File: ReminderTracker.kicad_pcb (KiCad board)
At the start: 2 copper layers, 92 x 150 mm, 23 parts, among them J1 External RTC, SW1 SW_Push, SW2 SW_Push, SW3 SW_Push, SW4 SW_Push, SW5 SW_Push, SW6 SW_Push, U1 XIAO-ESP32-C3-DIP

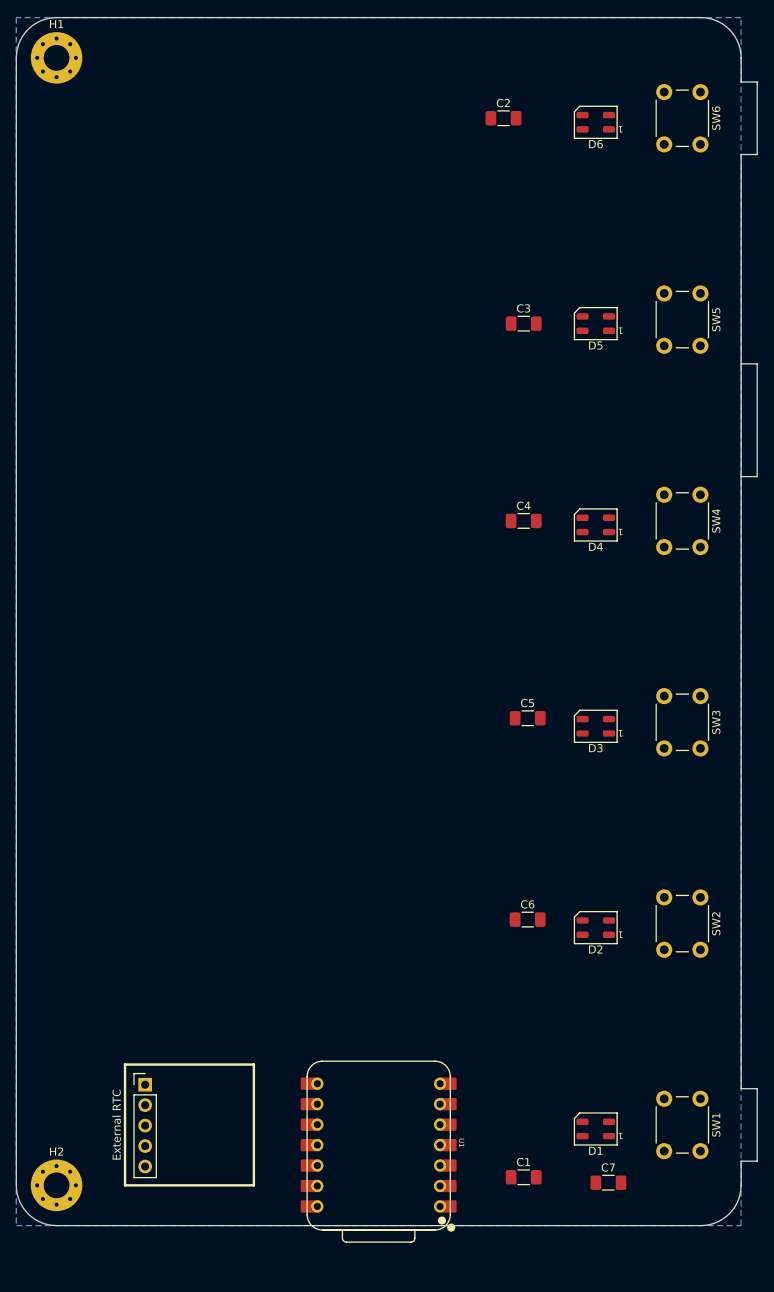
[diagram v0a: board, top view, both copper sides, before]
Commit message: R1
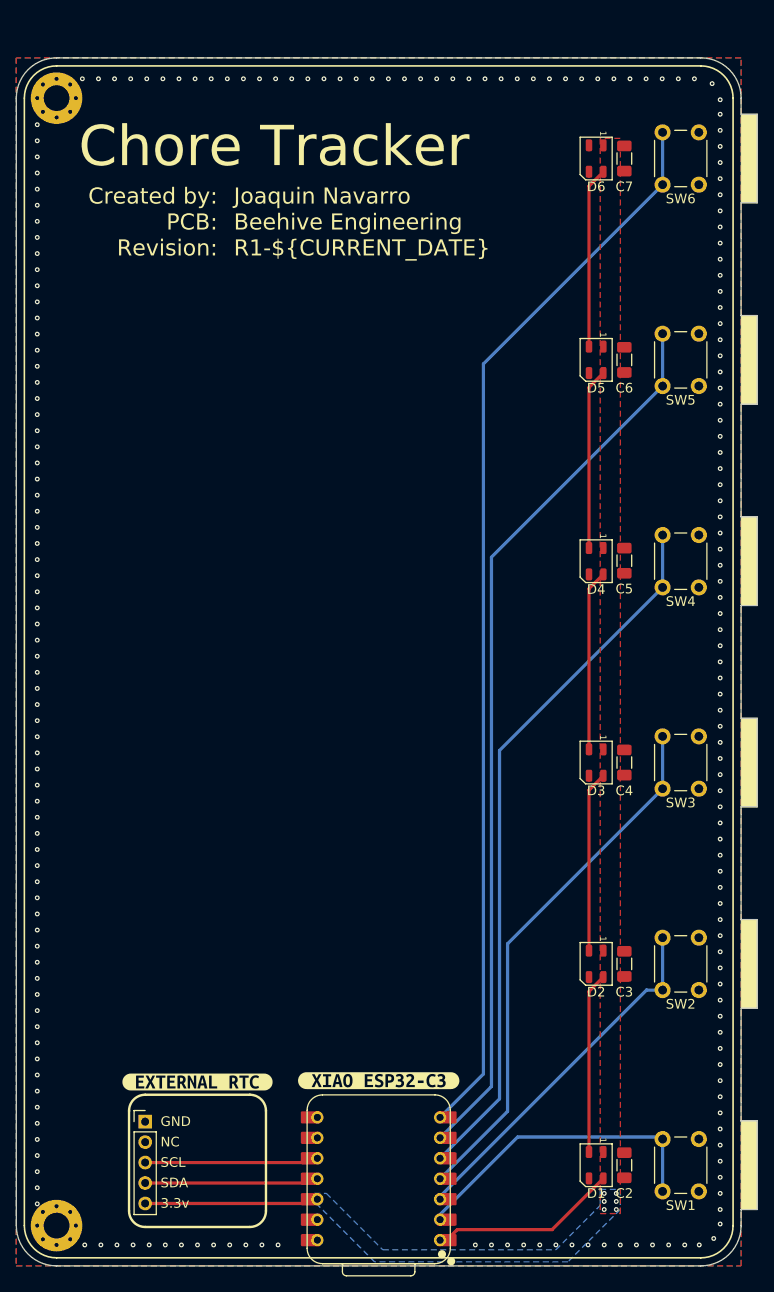
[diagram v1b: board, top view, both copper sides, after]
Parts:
- removed C1: 100pF, Capacitor_SMD:C_1206_3216Metric_Pad1.33x1.80mm_HandSolder
- added kibuzzard-69BB9782: G***, kibuzzard-69BB9782, F.Cu at (77.5, 157.2)
- added kibuzzard-69BB979E: G***, kibuzzard-69BB979E, F.Cu at (100.0, 157.0)
- moved C2 130.9 mm to (130.5, 167.5), turned to -90 degrees
- moved C7 127.2 mm to (130.5, 42.5), turned to -90 degrees
- moved C3 80.5 mm to (130.5, 142.5), turned to -90 degrees
- moved C6 70.5 mm to (130.5, 67.5), turned to -90 degrees
- moved C4 32.5 mm to (130.5, 117.5), turned to -90 degrees
- moved C5 22.9 mm to (130.5, 92.4), turned to -90 degrees
- moved SW1 5.00 mm to (139.8, 164.2)
- moved SW2 5.00 mm to (139.8, 139.2)
- moved SW3 5.00 mm to (139.8, 114.2)
- moved SW4 5.00 mm to (139.8, 89.2)
- moved SW5 5.00 mm to (139.8, 64.2)
- moved SW6 5.00 mm to (139.8, 39.2)
- moved H1 5.00 mm to (60.0, 35.0)
- moved H2 5.00 mm to (60.0, 175.0)
- moved J1 4.59 mm to (71.0, 162.1)
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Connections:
- C5 pad 1: Net-(D4-VDD) -> +3.3V
- C6 pad 1: Net-(D4-VDD) -> +3.3V
- C7 pad 1: Net-(D4-VDD) -> +3.3V
- D4 pad 1: Net-(D4-VDD) -> +3.3V
- D5 pad 1: Net-(D4-VDD) -> +3.3V
- D6 pad 1: Net-(D4-VDD) -> +3.3V
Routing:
- net BUTTON_6: track 0.00 -> 133.8 mm
- net BUTTON_5: track 0.00 -> 111.3 mm
- net BUTTON_4: track 0.00 -> 88.8 mm
- net BUTTON_3: track 0.00 -> 66.4 mm
- net BUTTON_2: track 0.00 -> 45.1 mm
- net BUTTON_1: track 0.00 -> 38.9 mm
- net LED_DATA: track 0.00 -> 22.6 mm
- net Net-(D1-DOUT): track 0.00 -> 22.5 mm
- net Net-(D2-DOUT): track 0.00 -> 22.5 mm
- net Net-(D5-DOUT): track 0.00 -> 22.5 mm
- net Net-(D4-DOUT): track 0.00 -> 22.5 mm
- net Net-(D3-DOUT): track 0.00 -> 22.5 mm
- net +3.3V: track 0.00 -> 21.6 mm, vias 0 -> 6
- net I2C_SDA: track 0.00 -> 20.8 mm
- net I2C_SCL: track 0.00 -> 20.8 mm
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- added copper zone on B.Cu, net +3.3V
- added copper zone on F.Cu, net +3.3V
- added copper zone on F.Cu, net GND
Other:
- outline, holes or cut-outs redrawn
- board text added: "3.3v"
- board text added: "Chore Tracker"
- board text added: "Created by: PCB: Revision:"
- board text added: "GND"
- board text added: "Joaquin Navarro Beehive Engineering ${REVISION}-${CURRENT_DATE}"
- board text added: "NC"
- board text added: "SCL"
- board text added: "SDA"
